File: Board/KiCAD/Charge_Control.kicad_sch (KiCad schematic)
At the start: 56 parts, among them Q1 AON7408, Q10 AON7407, Q2 AON7408, Q3 AON7408, Q4 AON7408, U1 BQ25730RSNR, U3 LTC2943CDD#PBF

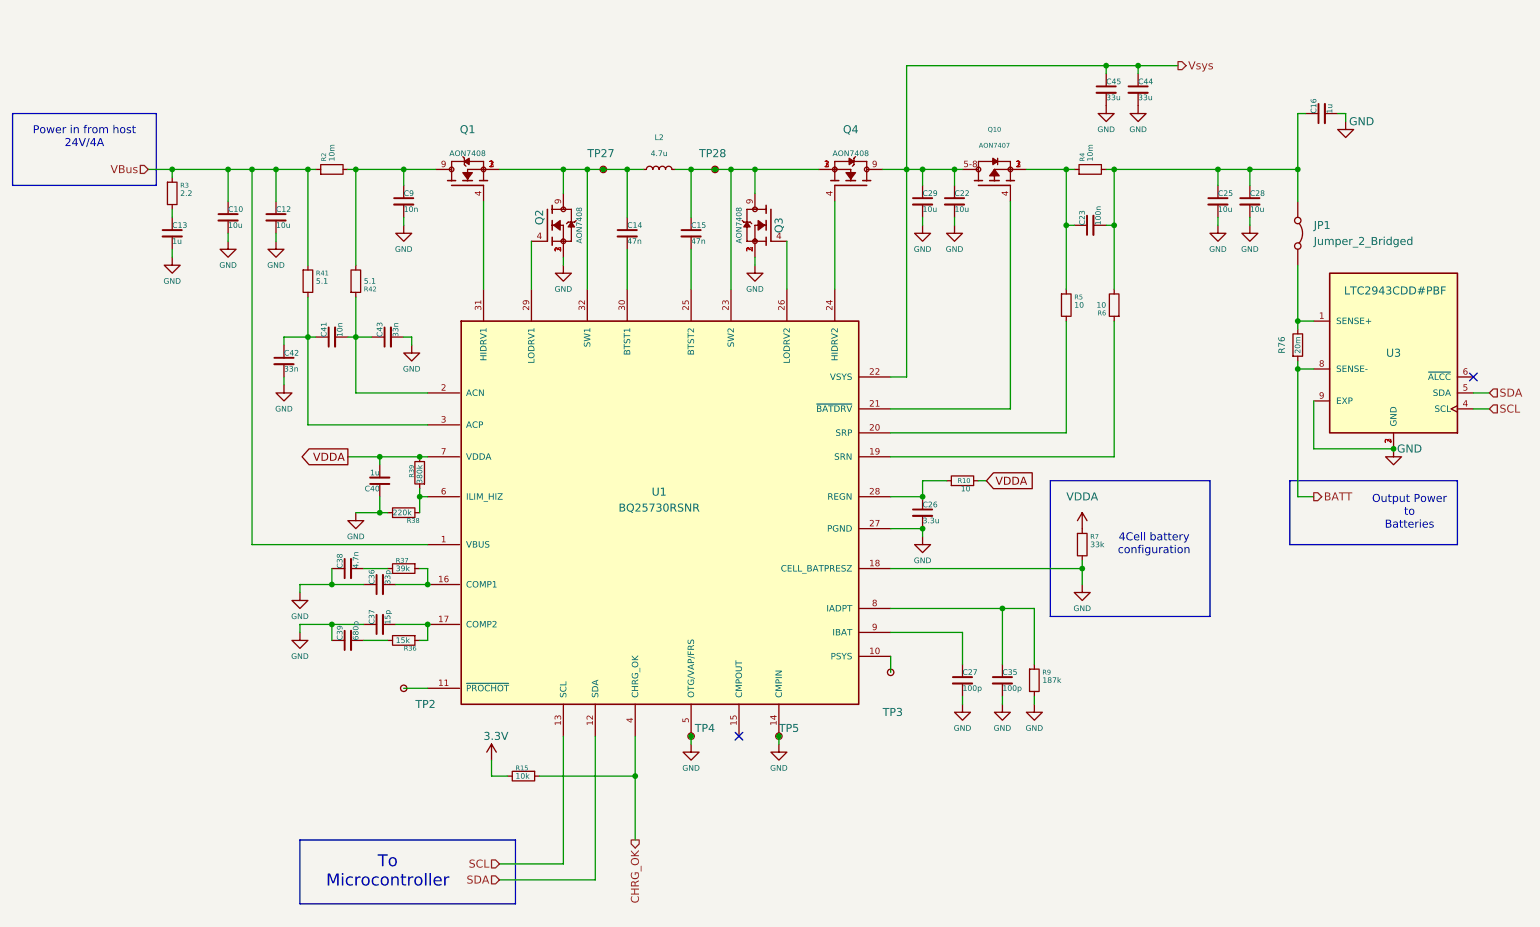
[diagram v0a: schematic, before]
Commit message: BOM Complete Need a Once Over Check
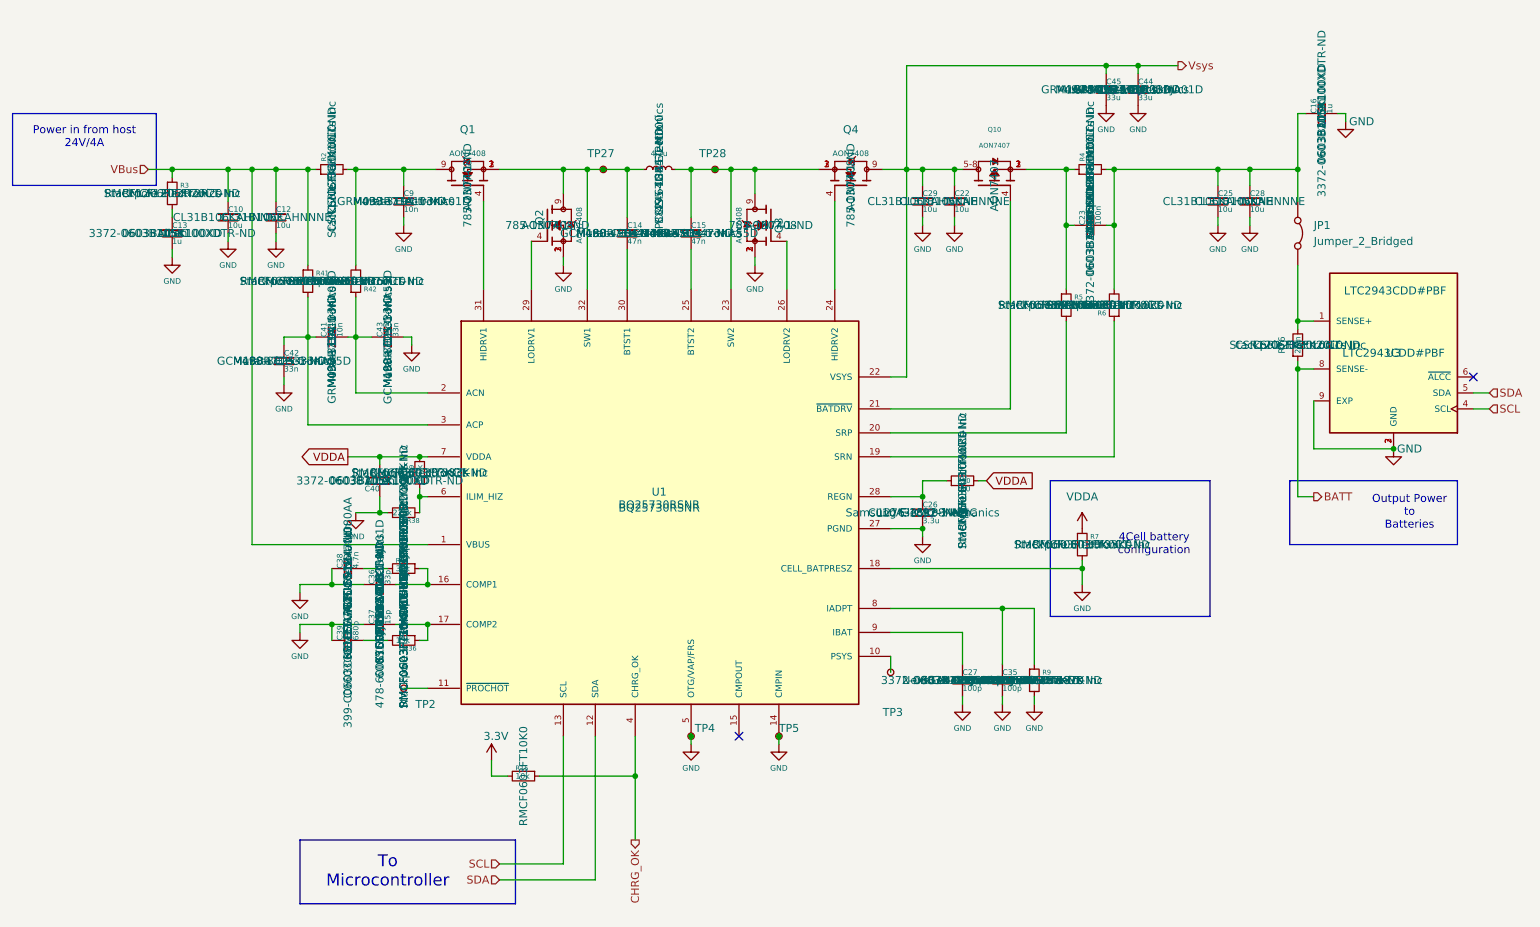
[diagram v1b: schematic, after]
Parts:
- C10, C12, C22, C25, C28, C29: MFR SAMSUNG -> Samsung Electro-Mechanics; MPN CL31A106KBHNNNE -> 1276-1804-1-ND; Package (none) -> CL31B106KAHNNNE
- C13, C16, C40: MFR (none) -> Aillen; MPN (none) -> 3372-0603B105K100XDTR-ND; Package (none) -> 0603B105K100XD
- C14, C15: MFR (none) -> Murata Electronics; MPN (none) -> 490-4934-1-ND; Package (none) -> GCM188R71H473KA55D
- C23: MFR (none) -> Aillen; MPN (none) -> 3372-0603B104K500XDTR-ND; Package (none) -> 0603B104K500XD
- C26: MFR (none) -> Samsung Electro-Mechanics; MPN (none) -> 1276-1892-1-ND; Package (none) -> CL10A335KP8NNNC
- C27, C35: MFR (none) -> NextGen Components; MPN (none) -> 3372-0603N101J500SDTR-ND; Package (none) -> 0603N101J500SD
- C36, C44, C45: MFR (none) -> Murata Electronics; MPN (none) -> 490-1415-1-ND; Package (none) -> GRM1885C1H330JA01D
- C37: MFR (none) -> KYOCERA AVX; MPN (none) -> 478-600S150JT250XT4KCT-ND; Package (none) -> 600S150JT250XT4K
- C38: MFR (none) -> TDK Corporation; MPN (none) -> 445-6912-1-ND; Package (none) -> CGA3E2C0G1H472J080AA
- C39: MFR (none) -> KEMET; MPN (none) -> 399-C0603C681F5GACTUCT-ND; Package (none) -> C0603C681F5GACTU
- C41, C9: MFR (none) -> Murata Electronics; MPN (none) -> 490-3194-1-ND; Package (none) -> GRM033R71A103KA01D
- C42, C43: MFR (none) -> Murata Electronics; MPN (none) -> 490-8025-1-ND; Package (none) -> GCM188R71H333KA55D
- L2: MFR (none) -> EPCOS - TDK Electronics; MPN (none) -> 495-1805-1-ND; Package (none) -> B82464G4472M000
- Q1, Q2, Q3, Q4: MPN (none) -> 785-1307-1-ND; Package (none) -> AON7408
- Q10: MPN AON7407 -> 785-1306-1-ND; Package (none) -> AON7407
- R10, R5, R6: MFR (none) -> Stackpole Electronics Inc; MPN (none) -> RMCF0603FT10R0CT-ND; Package (none) -> RMCF0603FT10R0
- R15: MPN RMCF0603FT10K0 -> RMCF0603FT10K0CT-ND; Package (none) -> RMCF0603FT10K0
- R2, R4: MFR (none) -> Stackpole Electronics Inc; MPN (none) -> CSR1206FK10L0CT-ND; Package (none) -> CSR1206FK10L0
- R3: MFR (none) -> Stackpole Electronics Inc; MPN (none) -> RMCF1206FT2R20CT-ND; Package (none) -> RMCF1206FT2R20
- R36: MFR (none) -> Stackpole Electronics Inc; MPN (none) -> RMCF0603FT15K0CT-ND; Package (none) -> RMCF0603FT15K0CT-ND
- R37: MFR (none) -> Stackpole Electronics Inc; MPN (none) -> RMCF0603JT39K0CT-ND; Package (none) -> RMCF0603JT39K0
- R38: MFR (none) -> Stackpole Electronics Inc; MPN (none) -> RMCF0603FT220KCT-ND; Package (none) -> RMCF0603FT220K
- R39: MFR (none) -> Stackpole Electronics Inc; MPN (none) -> RMCF0603FT383KCT-ND; Package (none) -> RMCF0603FT383K
- R41, R42: MFR (none) -> Stackpole Electronics Inc; MPN (none) -> RMCF0603FT5R10CT-ND; Package (none) -> RMCF0603FT5R10
- R7: MFR (none) -> Stackpole Electronics Inc; MPN (none) -> RMCF0603FT33K0CT-ND; Package (none) -> RMCF0603FT33K0
- R76: MFR (none) -> Stackpole Electronics Inc; MPN (none) -> CSR1206FK20L0CT-ND; Package (none) -> CSR1206FK20L0
- R9: MFR (none) -> Stackpole Electronics Inc; MPN (none) -> RMCF0603FT187KCT-ND; Package (none) -> RMCF0603FT187K
- U1: Package (none) -> BQ25730RSNR
- U3: Package (none) -> LTC2943CDD#PBF

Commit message: Updated schematic
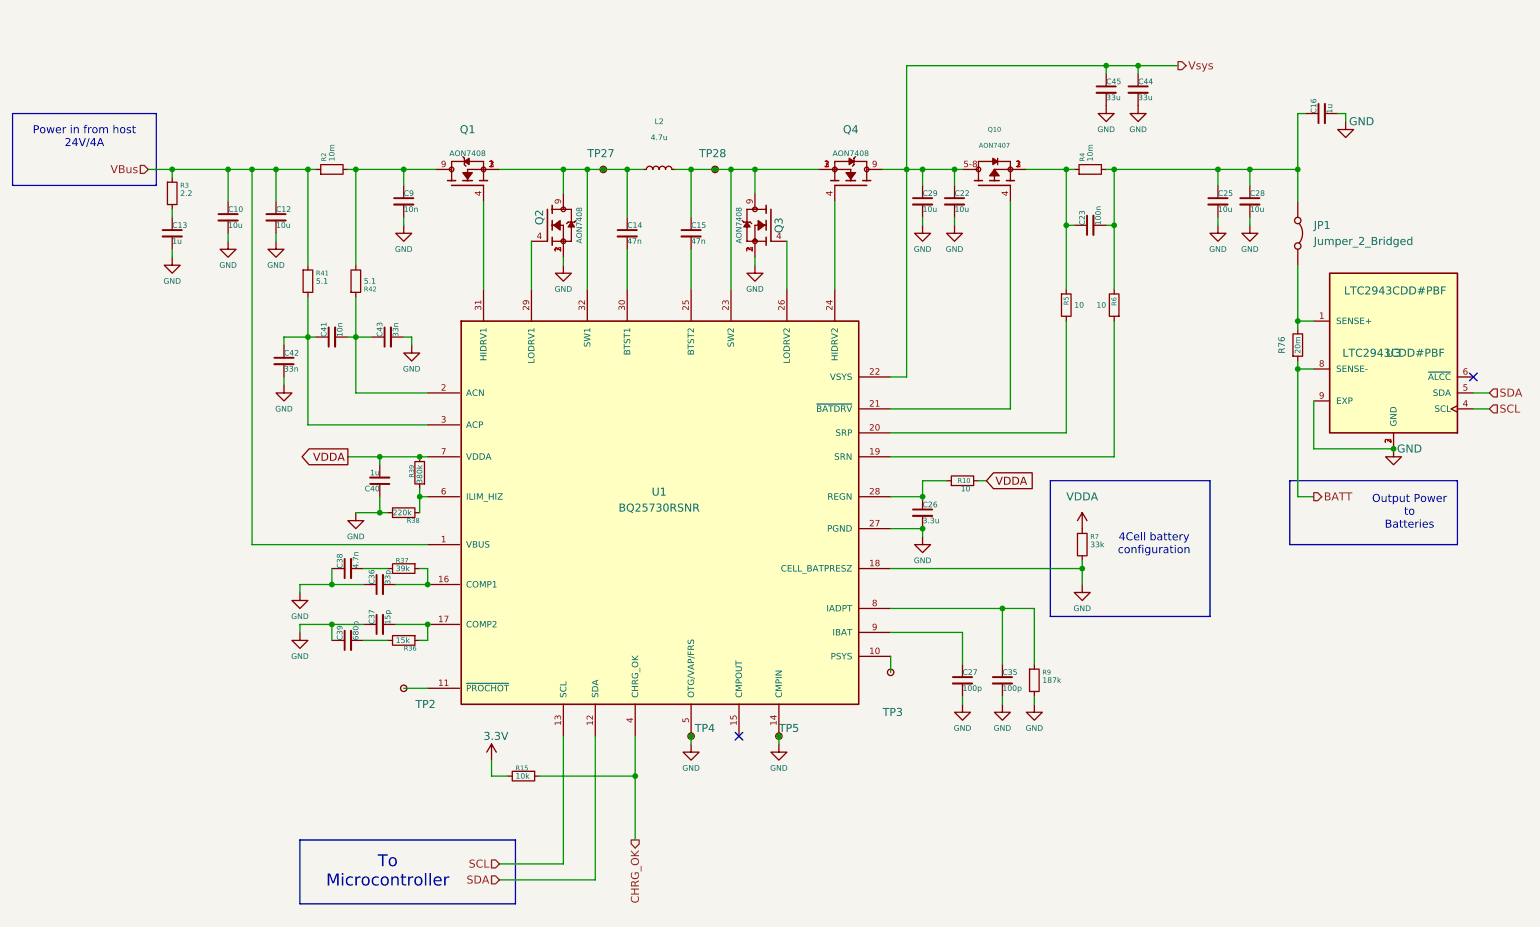
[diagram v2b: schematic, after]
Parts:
- C26: MFR Samsung Electro-Mechanics -> (none)
- C36: Package GRM1885C1H330JA01D -> (none)
- C42: MFR Murata Electronics -> (none)
- C43: MFR Murata Electronics -> urata Electronics
- L2: MFR EPCOS - TDK Electronics -> (none)
- R3: MPN RMCF1206FT2R20CT-ND -> (none)
